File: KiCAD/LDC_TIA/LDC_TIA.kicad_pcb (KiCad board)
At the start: 2 copper layers, 22 parts, among them J1 Conn_01x02_Pin, J2 54-00166, J5 Conn_01x07_Pin, Q1 BC817, U2 LM7805_TO220, U3 OPA2197xD, U4 LTC1044

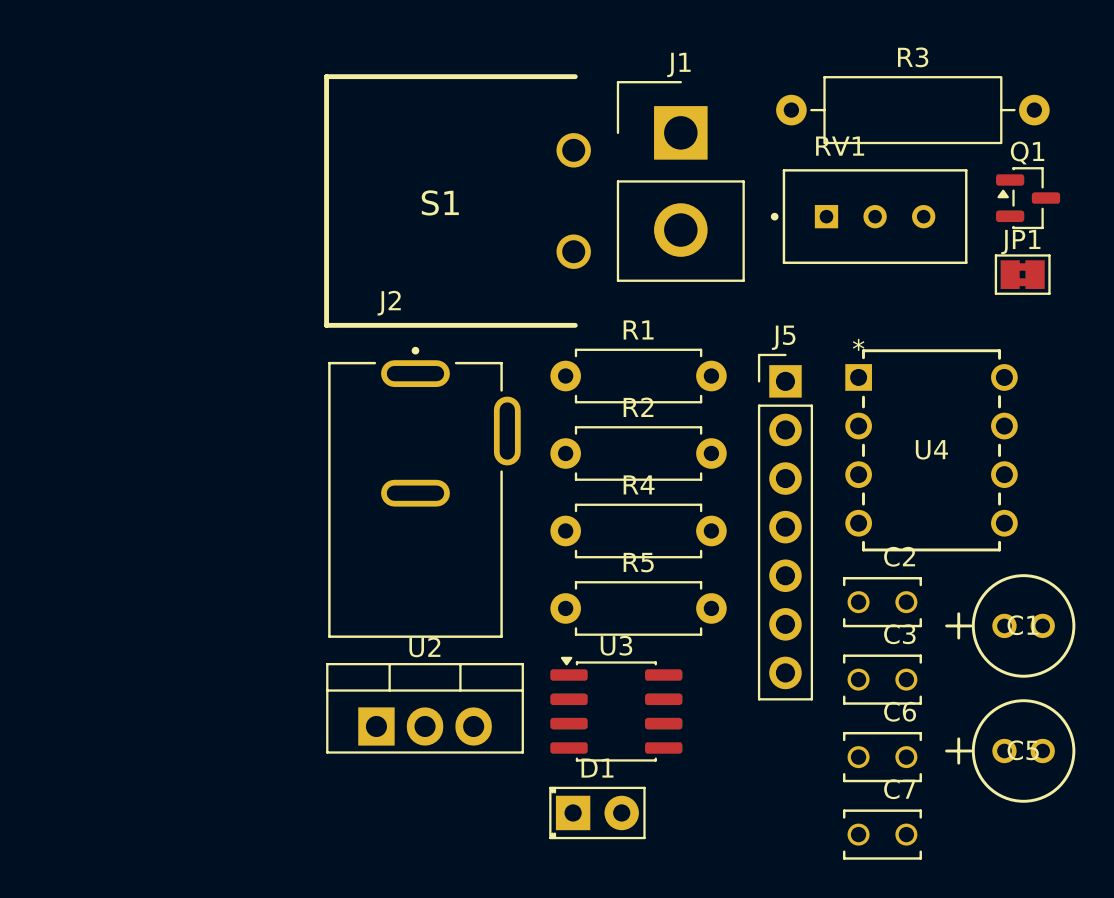
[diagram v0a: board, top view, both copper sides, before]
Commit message: PCB layout
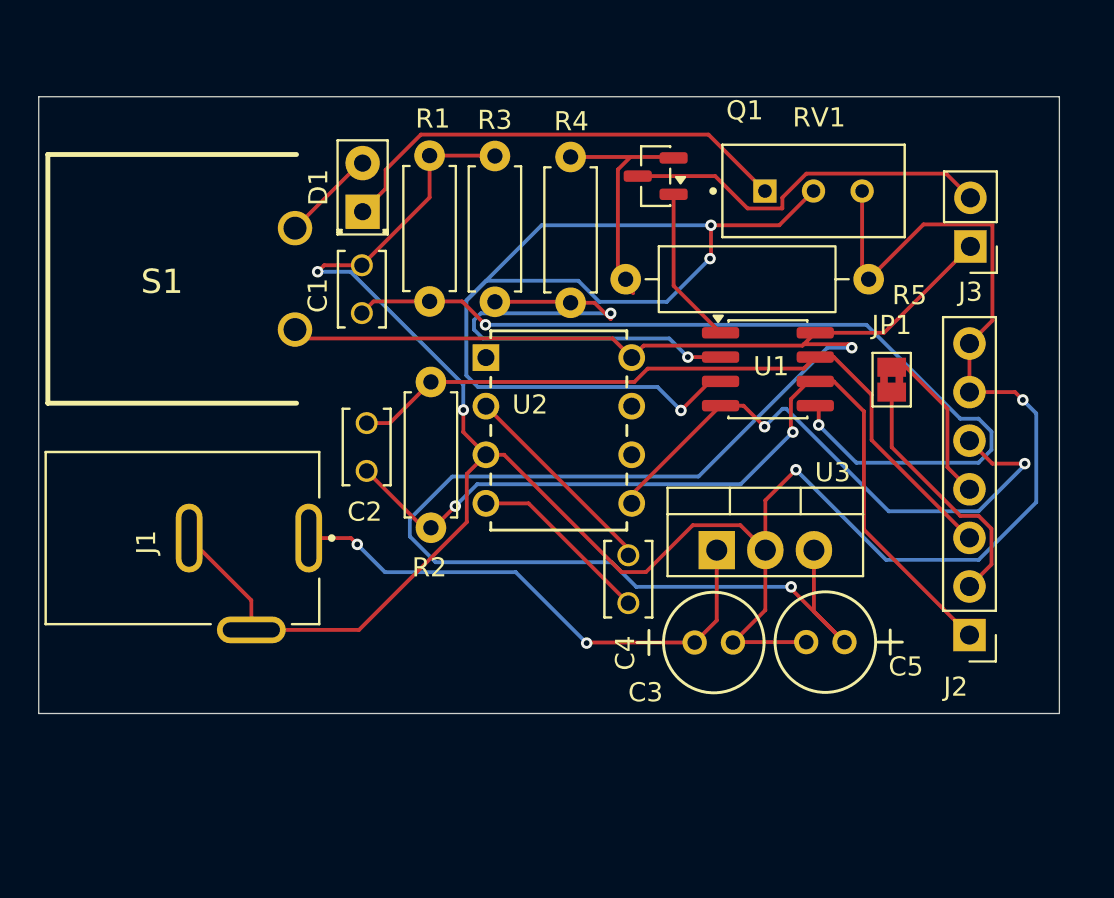
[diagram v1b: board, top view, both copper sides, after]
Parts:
- removed C6: 10pF, FOOTPRINTS:CAPRB250W50L400T250H550
- J3: renamed from J1; footprint Connector_Samtec_HPM_THT:Samtec_HPM-02-01-x-S_Straight_1x02_Pitch5.08mm -> Connector_PinHeader_2.54mm:PinHeader_1x02_P2.54mm_Vertical
- moved C1 39.4 mm to (131.6, 92.2), turned to 90 degrees
- moved D1 33.3 mm to (131.6, 88.2), turned to 90 degrees
- moved C2 28.2 mm to (131.8, 100.5), turned to 90 degrees
- moved U3 20.0 mm to (150.1, 105.9)
- moved U1 19.6 mm to (152.8, 96.4)
- moved U2 19.5 mm to (138.0, 95.8)
- moved Q1 19.5 mm to (146.9, 86.3), turned to 180 degrees
- moved C3 17.2 mm to (149.0, 110.7)
- moved J2 16.4 mm to (163.3, 110.3), turned to 180 degrees
- moved J3 16.3 mm to (163.4, 90.0), turned to 180 degrees
- moved S1 15.1 mm to (128.1, 91.7)
- moved C4 14.3 mm to (145.5, 107.4), turned to -90 degrees
- moved R1 13.9 mm to (135.1, 92.9), turned to 90 degrees
- moved R5 12.4 mm to (145.3, 91.7)
- moved J1 12.1 mm to (122.5, 105.2), turned to -90 degrees
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- renumbered C7 to C1, C5 to C3, C3 to C4, C1 to C5, J2 to J1, J5 to J2, R4 to R1, R5 to R2, R1 to R3, R2 to R4, R3 to R5, U3 to U1, U4 to U2, U2 to U3
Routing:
- net GND: track 0.00 -> 129.7 mm, vias 0 -> 4
- net /+VCC: track 0.00 -> 99.2 mm, vias 0 -> 2
- net Net-(U1A-+): track 0.00 -> 55.4 mm, vias 0 -> 3
- net Net-(U1B-+): track 0.00 -> 48.1 mm, vias 0 -> 2
- net /CATHODE: track 0.00 -> 46.2 mm, vias 0 -> 2
- net /VOUT: track 0.00 -> 38.2 mm
- net /-VCC: track 0.00 -> 30.5 mm, vias 0 -> 2
- net Net-(U1A--): track 0.00 -> 28.0 mm, vias 0 -> 2
- net /VI: track 0.00 -> 27.8 mm, vias 0 -> 2
- net Net-(D1-K): track 0.00 -> 24.5 mm
- net Net-(J3-Pin_2): track 0.00 -> 19.7 mm
- net /ANODE: track 0.00 -> 13.4 mm
- net Net-(Q1-E): track 0.00 -> 12.2 mm
- net Net-(U2-CAP+): track 0.00 -> 10.9 mm
- net Net-(U2-CAP-): track 0.00 -> 9.61 mm
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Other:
- board outline added: 53.4 x 32.2 mm
